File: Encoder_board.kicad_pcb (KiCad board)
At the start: 2 copper layers, 70 x 70 mm, 76 parts, among them J1 Conn_01x05_Socket_RS485, J2 CAN_OUT, J3 Conn_01x05_Socket_Encoder4, J4 Conn_01x05_Socket_Encoder1, J5 Conn_01x05_Socket_Encoder2, J6 Conn_01x05_Socket_Encoder5, J7 ST-Link_pinsocket, J8 Conn_01x05_Socket_Encoder3, SW1 SW_Boot, SW2 SW_Reset, SW3 SW_DIP_x02_CANnum, SW4 SW_User, U1 XT60_M, U2 UTRS485G-S08-R, U3 UTRS485G-S08-R, U4 MCP2562-E-P, U5 BA05CC0FP, U6 BA033CC0FP, U7 STM32G431KBTx

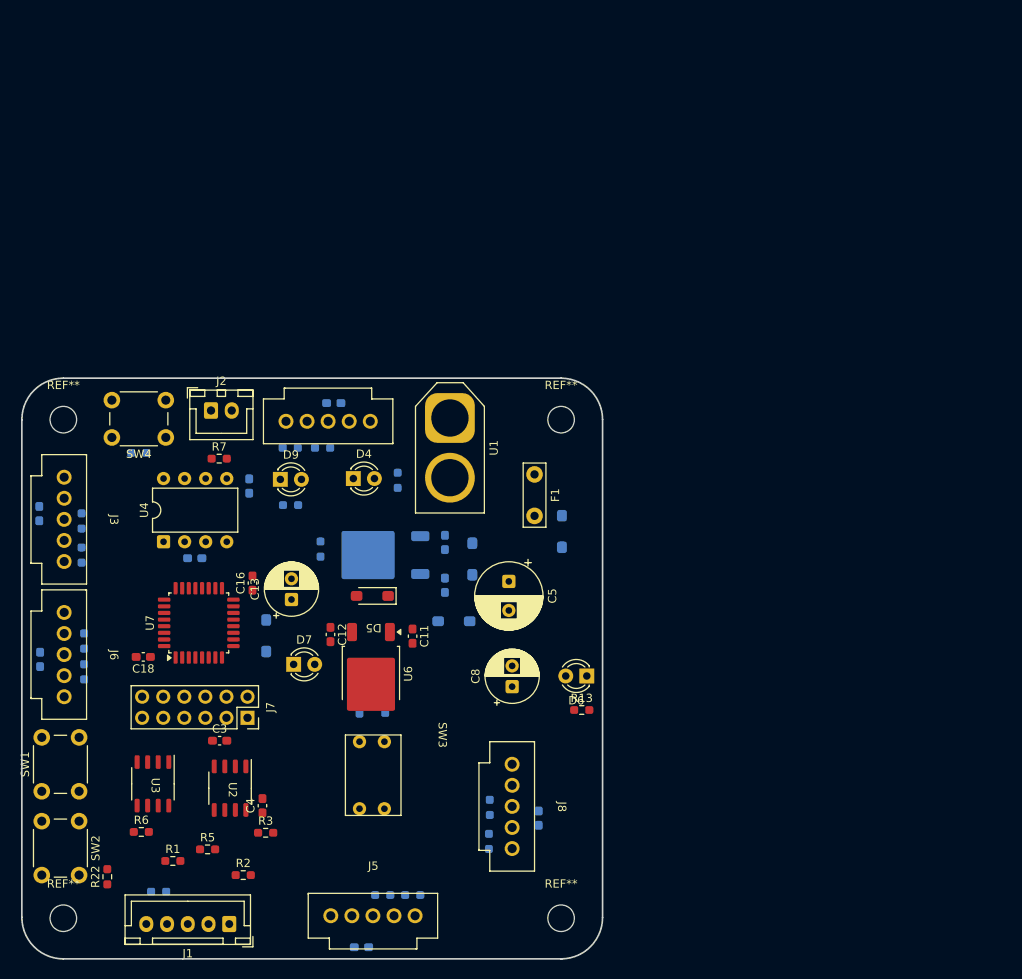
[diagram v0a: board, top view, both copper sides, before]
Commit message: 配線終了。あとはシルク
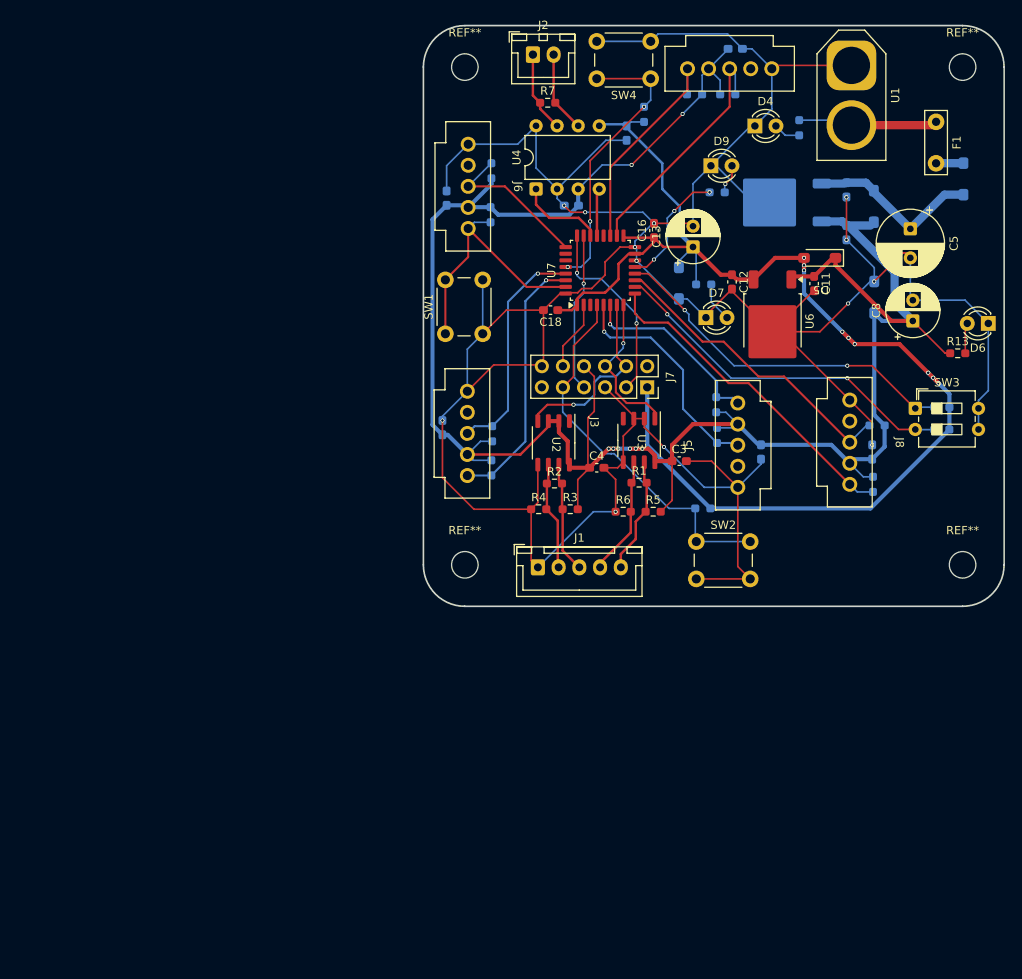
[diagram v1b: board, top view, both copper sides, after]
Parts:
- R22: moved to B.Cu
- R4: moved to F.Cu
- SW3: footprint mylib:DIP_sw_02_9.7_6.7 -> Button_Switch_THT:SW_DIP_SPSTx02_Slide_6.7x6.64mm_W7.62mm_P2.54mm_LowProfile
- moved R22 84.4 mm to (142.2, 115.7), turned to 180 degrees
- moved SW2 81.7 mm to (141.4, 119.7), turned to 0 degrees
- moved R24 77.7 mm to (171.0, 106.2), turned to 180 degrees
- moved C14 76.7 mm to (149.2, 108.9), turned to -90 degrees
- moved R23 76.1 mm to (171.0, 103.5), turned to 180 degrees
- moved R16 75.0 mm to (116.7, 75.0)
- moved J6 74.5 mm to (119.4, 76.9)
- moved C15 74.1 mm to (111.3, 78.3)
- moved R18 73.7 mm to (116.6, 80.3)
- moved SW1 73.5 mm to (111.2, 94.7)
- moved SW3 73.4 mm to (167.8, 103.6), turned to 0 degrees
- moved R25 73.3 mm to (135.1, 68.2), turned to 90 degrees
- moved SW4 72.7 mm to (135.9, 63.9)
- moved R1 72.4 mm to (134.5, 112.6)
- moved U3 71.7 mm to (134.3, 107.7)
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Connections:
- R22 pad 1: +5V -> +3V3
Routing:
- net GND: track 0.00 -> 406.2 mm, vias 0 -> 13
- net +5V: track 0.00 -> 264.2 mm, vias 0 -> 8
- net +3V3: track 0.00 -> 161.0 mm, vias 0 -> 9
- net RESET: track 0.00 -> 46.0 mm
- net CAN_num1: track 0.00 -> 43.3 mm, vias 0 -> 2
- net CAN_num2: track 0.00 -> 43.3 mm, vias 0 -> 2
- net En3_B: track 0.00 -> 40.4 mm
- net En3_A: track 0.00 -> 37.2 mm
- net User_button: track 0.00 -> 34.5 mm, vias 0 -> 3
- net En4_B: track 0.00 -> 31.5 mm, vias 0 -> 1
- net En5_B: track 0.00 -> 31.5 mm
- net En1_A: track 0.00 -> 29.1 mm
- net En2_A: track 0.00 -> 27.8 mm, vias 0 -> 1
- net En4_A: track 0.00 -> 27.5 mm, vias 0 -> 1
- net En1_B: track 0.00 -> 27.1 mm
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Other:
- outline, holes or cut-outs redrawn
